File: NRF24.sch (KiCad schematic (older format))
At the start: 47 parts, among them J1 Conn_ARM_JTAG_SWD_10, J2 SMA, Q1 AO3401A, Q2 AO3401A, Q3 AO3401A, U1 SI7021, U2 STM32L031G6Ux, U3 nRF24L01P, Y1 16MHz

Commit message: Firmware Blinky Test
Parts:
- BT1: Mouser (none) -> 534-1060TR
- J1: Mouser (none) -> 855-M50-3610542R
- J2: Mouser (none) -> 200-SMAJPHSTEM1
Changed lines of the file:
@@
 F 2 "Battery:BatteryHolder_Keystone_1060_1x2032" V 900 1360 50  0001 C CNN
 F 3 "~" V 900 1360 50  0001 C CNN
+F 4 "534-1060TR" H 900 1300 50  0001 C CNN "Mouser"
 	1    900  1300
 	1    0    0    -1
@@
 F 2 "Connector_PinHeader_1.27mm:PinHeader_2x05_P1.27mm_Vertical_SMD" H 1400 5100 50  0001 C CNN
 F 3 "http://infocenter.arm.com/help/topic/com.arm.doc.ddi0314h/DDI0314H_coresight_components_trm.pdf" V 1050 3850 50  0001 C CNN
+F 4 "855-M50-3610542R" H 1400 5100 50  0001 C CNN "Mouser"
 	1    1400 5100
 	1    0    0    -1
@@
 F 2 "ak:SMA_Samtec_SMA-J-P-H-ST-EM1_EdgeMount" H 10700 2100 50  0001 C CNN
 F 3 " ~" H 10700 2100 50  0001 C CNN
+F 4 "200-SMAJPHSTEM1" H 10700 2100 50  0001 C CNN "Mouser"
 	1    10700 2100
 	1    0    0    -1

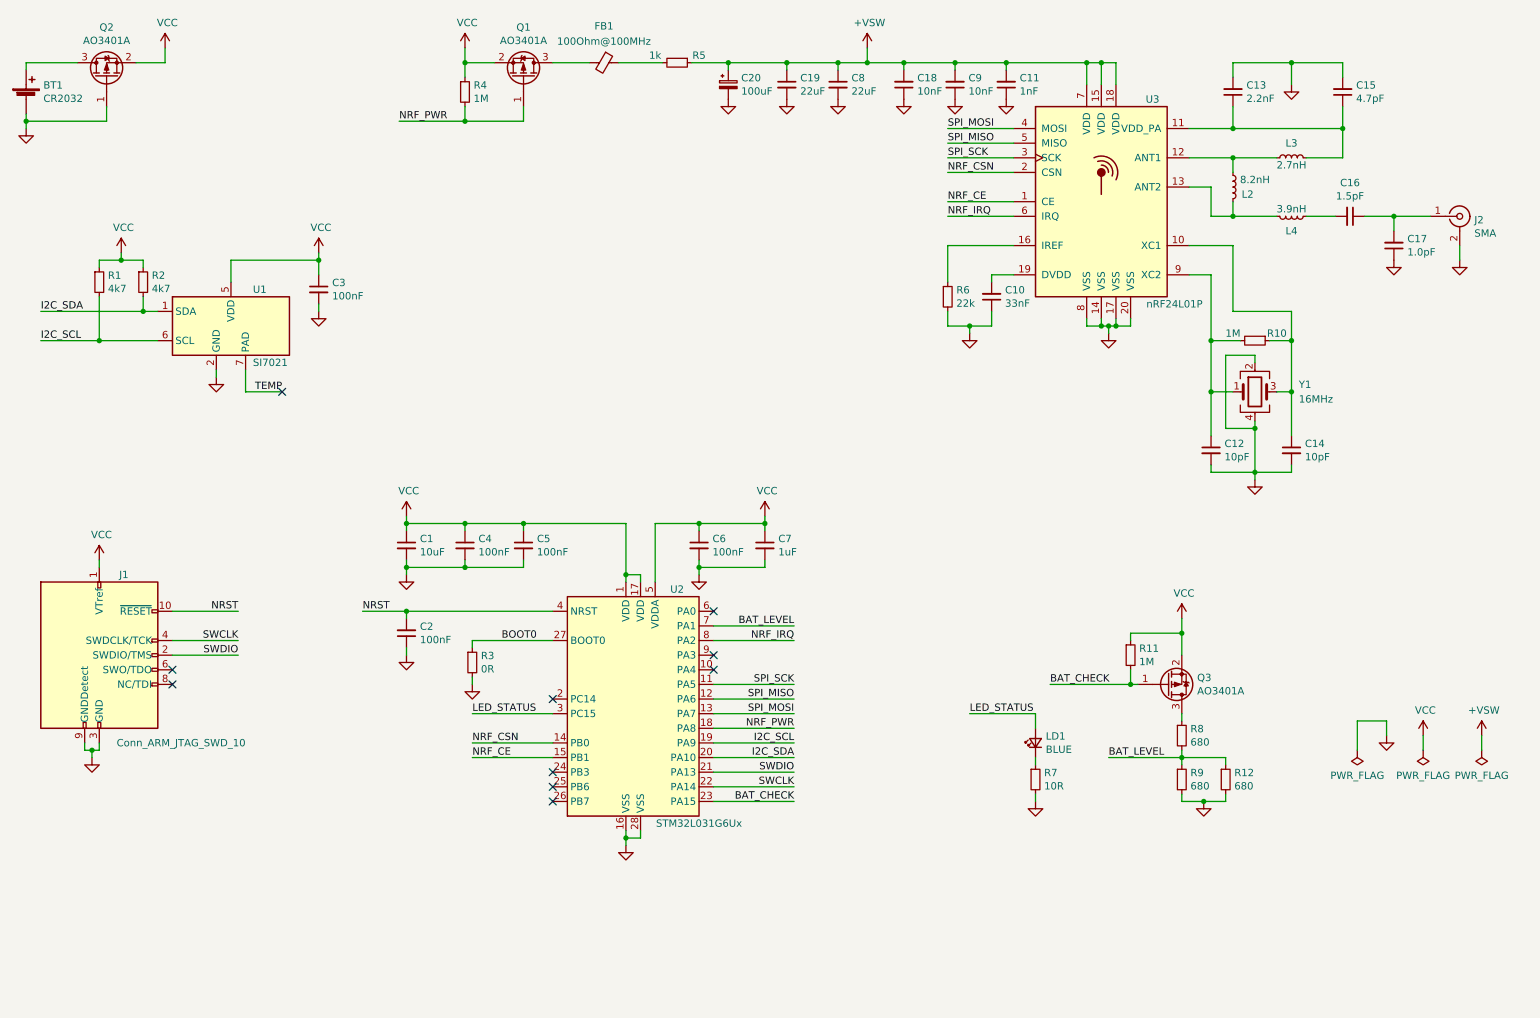
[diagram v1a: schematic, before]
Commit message: Updated schematic
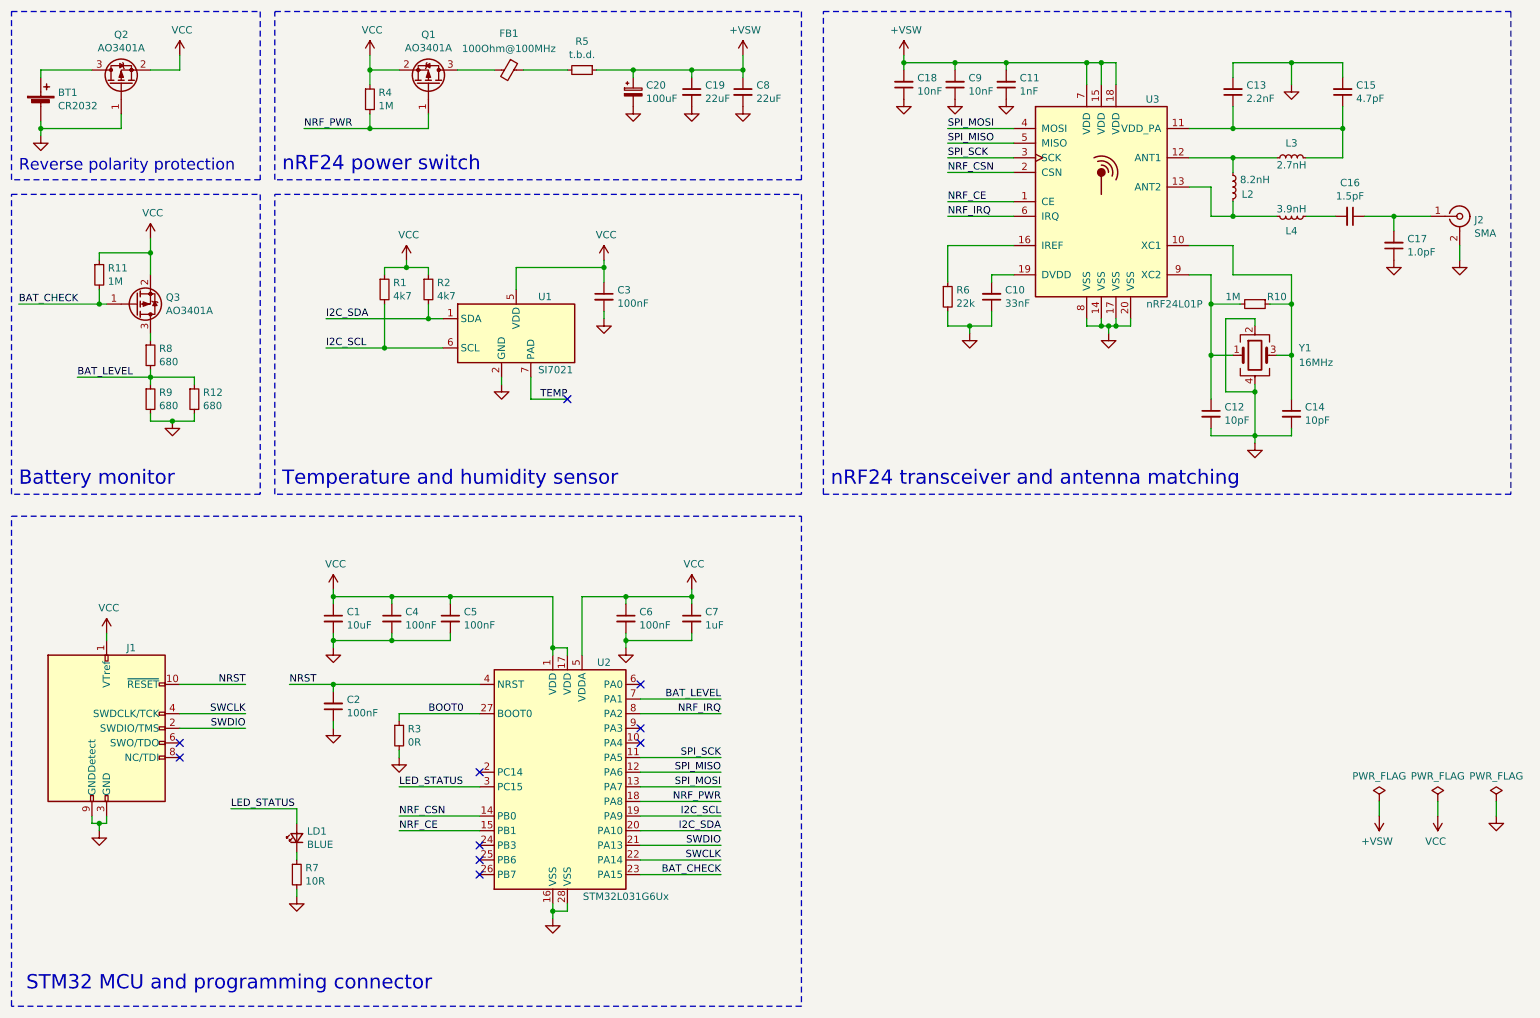
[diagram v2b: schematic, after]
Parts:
- R5: value 1k -> t.b.d.
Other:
- note added: "Battery monitor"
- note added: "Reverse polarity protection"
- note added: "STM32 MCU and programming connector"
- note added: "Temperature and humidity sensor"
- note added: "nRF24 power switch"
- note added: "nRF24 transceiver and antenna matching"
- moved on the sheet: BT1, C1, C12, C14, C19, C2, C20, C3, C4, C5, C6, C7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
